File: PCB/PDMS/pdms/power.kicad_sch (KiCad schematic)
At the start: 53 parts, among them IC1 BD50FD0WHFP-TR, IC10 LDO40LPU50RY, IC11 MP2332HGTL-P, IC14 LDO40LPU50RY, IC3 LDO40LPU33RY, Q1 AO3401A, Q11 AO3401A

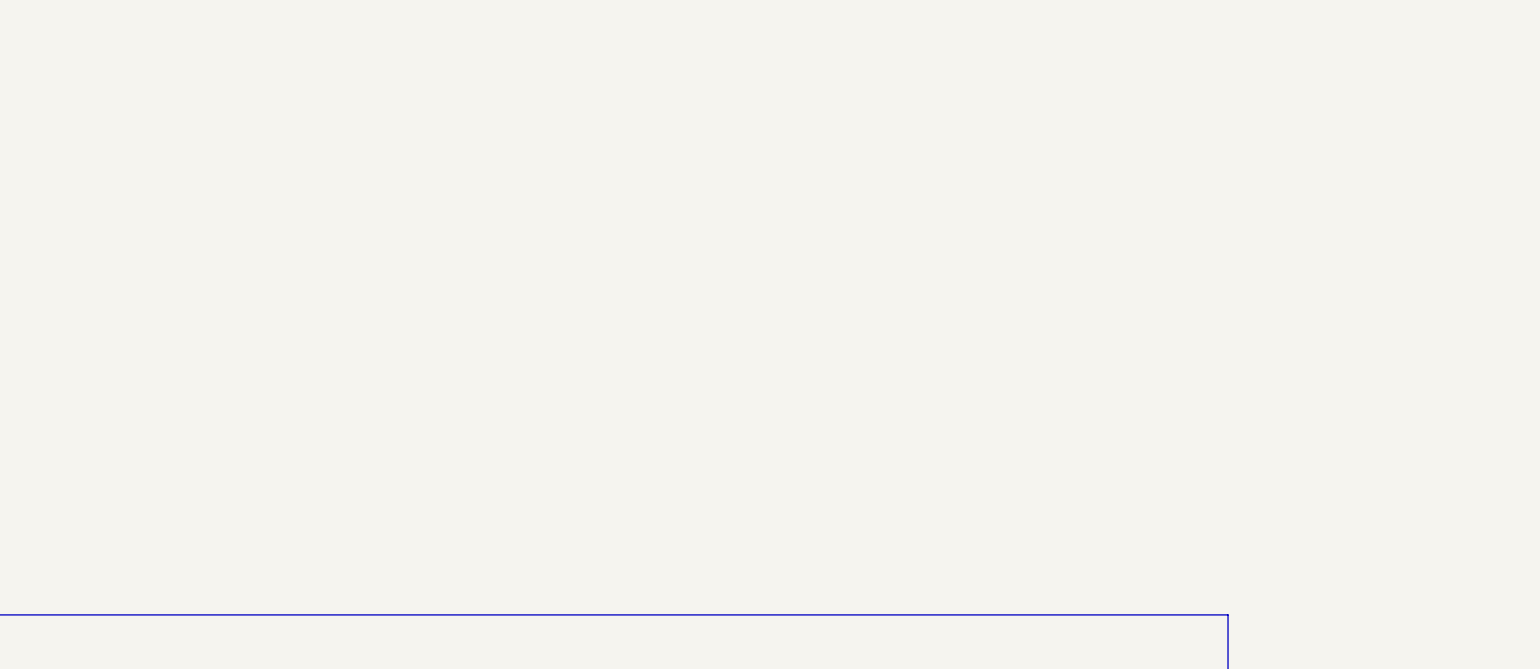
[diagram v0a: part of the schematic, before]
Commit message: Ver 4.2 ready + BTS50025 test board
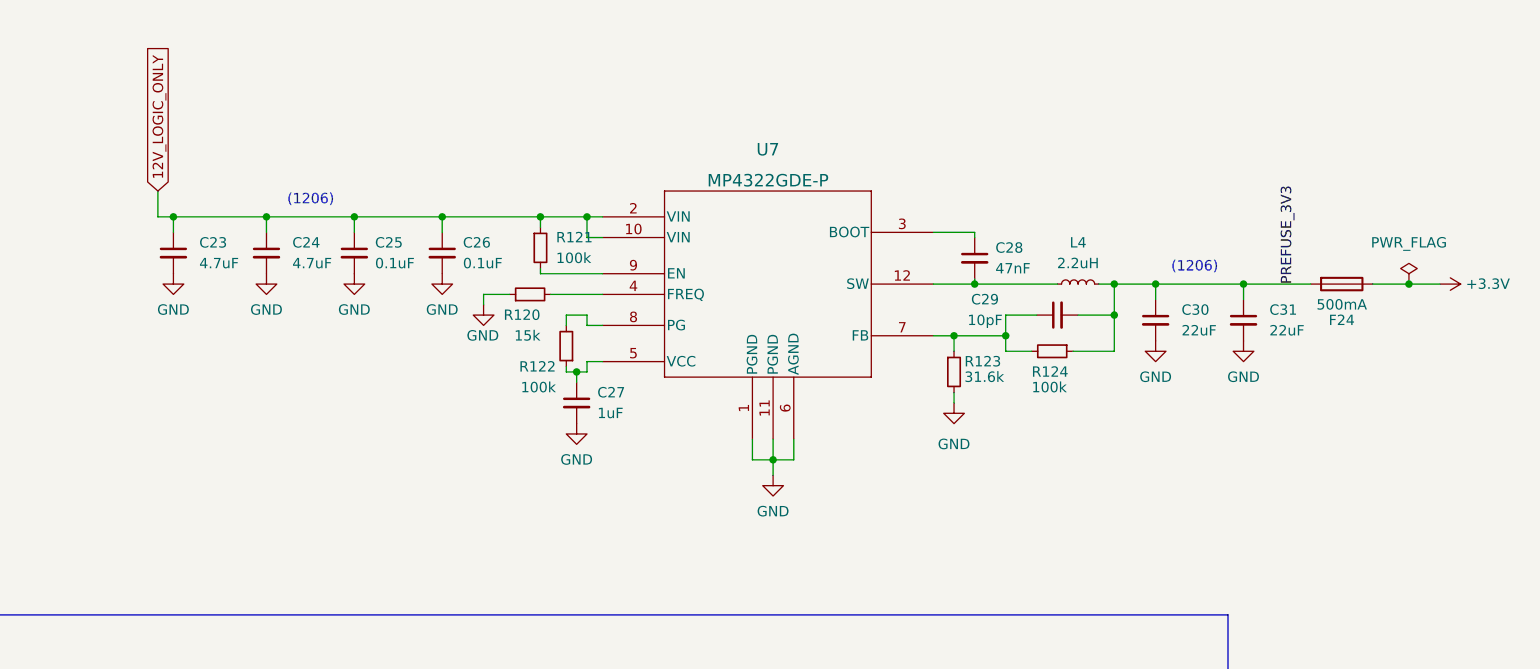
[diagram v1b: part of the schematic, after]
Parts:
- added C23, C24: 4.7uF, Capacitor_SMD:C_1206_3216Metric, symbol Device:C_Small
- added C25, C26: 0.1uF, Capacitor_SMD:C_0805_2012Metric, symbol Device:C_Small
- added C27: 1uF, Resistor_SMD:R_0402_1005Metric, symbol Device:C_Small
- added C28: 47nF, Resistor_SMD:R_0402_1005Metric, symbol Device:C_Small
- added C29: 10pF, Resistor_SMD:R_0402_1005Metric, symbol Device:C_Small
- added C30, C31: 22uF, Capacitor_SMD:C_1206_3216Metric, symbol Device:C_Small
- added F24: 500mA, Fuse:Fuse_0805_2012Metric, symbol Device:Fuse
- added L4: 2.2uH, Inductor_SMD:L_Vishay_IHLP-1616, symbol Device:L_Small
- added R120: 15k, Resistor_SMD:R_0402_1005Metric, symbol Device:R_Small
- added R121, R122, R124: 100k, Resistor_SMD:R_0402_1005Metric, symbol Device:R_Small
- added R123: 31.6k, Resistor_SMD:R_0402_1005Metric, symbol Device:R_Small
- added U7: MP4322GDE-P, PDMS_Additional:QFN-12_MP4322_MNP, symbol pdms_additional:MP4322GDE-P
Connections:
- net +3.3V: now also F24.1
- net 12V_LOGIC_ONLY: now also C23.1, C24.1, C25.1, C26.1, R121.1, U7.10 (VIN), U7.2 (VIN)
- net GND: now also C23.2, C24.2, C25.2, C26.2, C27.2, C30.2, C31.2, R120.1, R123.2, U7.1 (PGND), U7.11 (PGND), U7.6 (AGND)
- net PREFUSE_3V3: now also C29.2, C30.1, C31.1, F24.2, L4.2, R124.1
- new net: C29.1, R123.1, R124.2, U7.7 (FB)
- new net: R121.2, U7.9 (EN)
- new net: C28.2, L4.1, U7.12 (SW)
- new net: C28.1, U7.3 (BOOT)
- new net: R120.2, U7.4 (FREQ)
- new net: C27.1, R122.1, U7.5 (VCC)
- new net: R122.2, U7.8 (PG)
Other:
- note added: "(1206)"

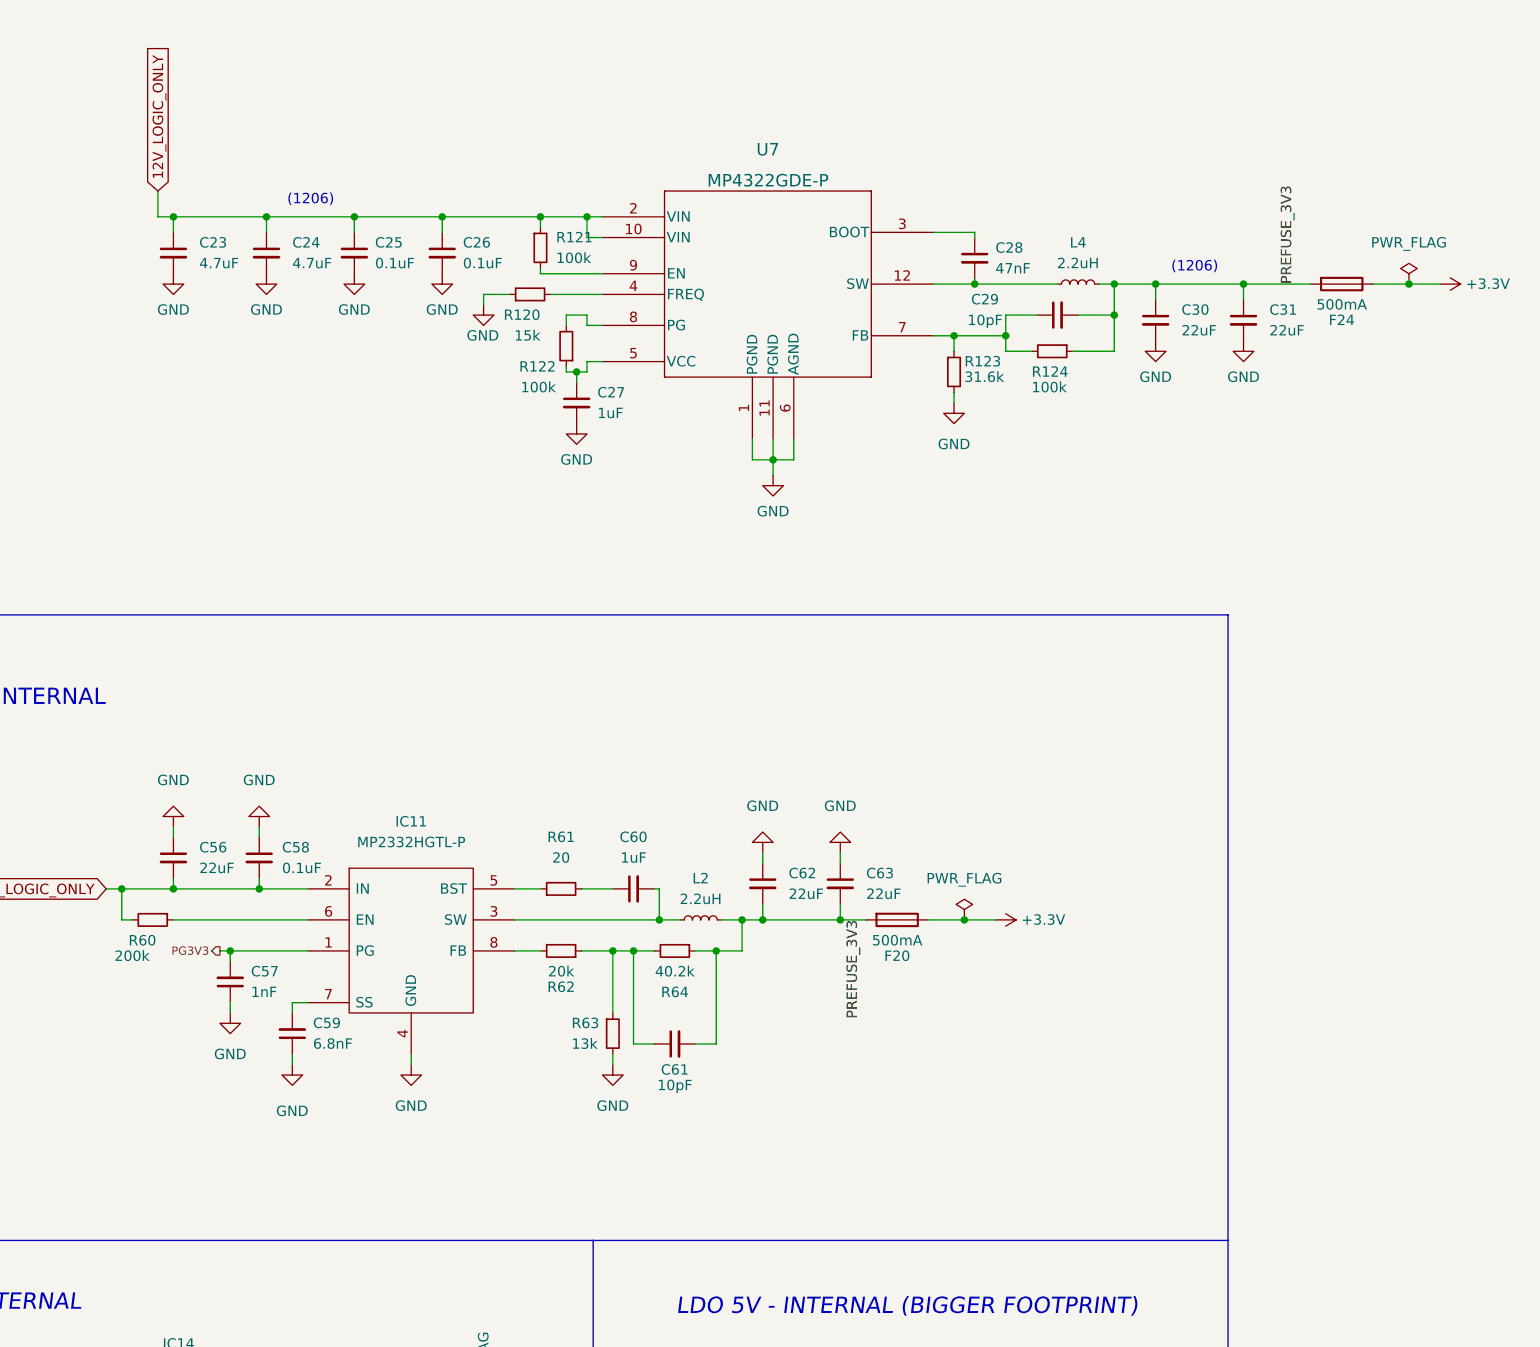
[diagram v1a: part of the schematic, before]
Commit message: Minor changes in overall schematics & MP4322 scheamtics
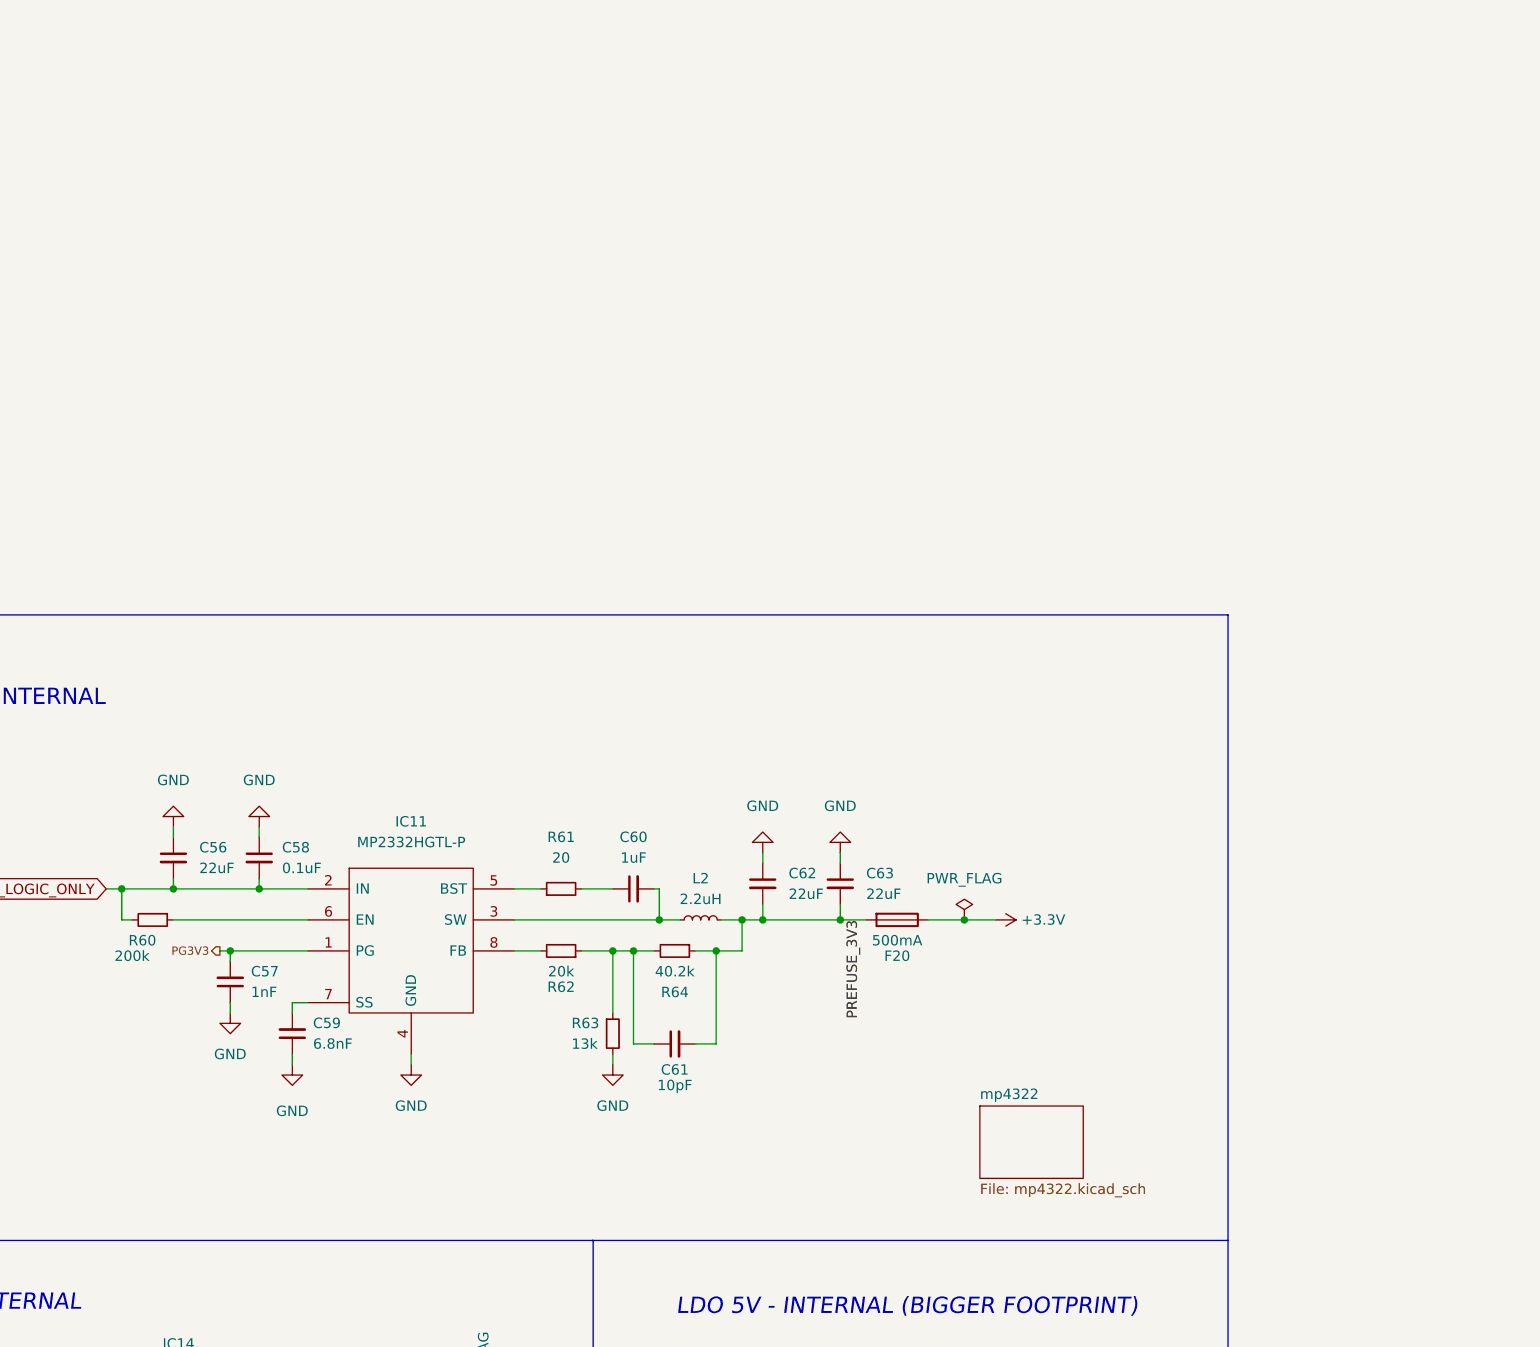
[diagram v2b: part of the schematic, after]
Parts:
- removed C23, C24: 4.7uF, Capacitor_SMD:C_1206_3216Metric, symbol Device:C_Small
- removed C25, C26: 0.1uF, Capacitor_SMD:C_0805_2012Metric, symbol Device:C_Small
- removed C27: 1uF, Resistor_SMD:R_0402_1005Metric, symbol Device:C_Small
- removed C28: 47nF, Resistor_SMD:R_0402_1005Metric, symbol Device:C_Small
- removed C29: 10pF, Resistor_SMD:R_0402_1005Metric, symbol Device:C_Small
- removed C30, C31: 22uF, Capacitor_SMD:C_1206_3216Metric, symbol Device:C_Small
- removed F24: 500mA, Fuse:Fuse_0805_2012Metric, symbol Device:Fuse
- removed L4: 2.2uH, Inductor_SMD:L_Vishay_IHLP-1616, symbol Device:L_Small
- removed R120: 15k, Resistor_SMD:R_0402_1005Metric, symbol Device:R_Small
- removed R121, R122, R124: 100k, Resistor_SMD:R_0402_1005Metric, symbol Device:R_Small
- removed R123: 31.6k, Resistor_SMD:R_0402_1005Metric, symbol Device:R_Small
- removed U7: MP4322GDE-P, PDMS_Additional:QFN-12_MP4322_MNP, symbol pdms_additional:MP4322GDE-P
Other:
- added sheet mp4322 (mp4322.kicad_sch)
- note removed: "(1206)"
